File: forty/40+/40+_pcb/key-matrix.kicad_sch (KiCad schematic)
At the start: 48 parts

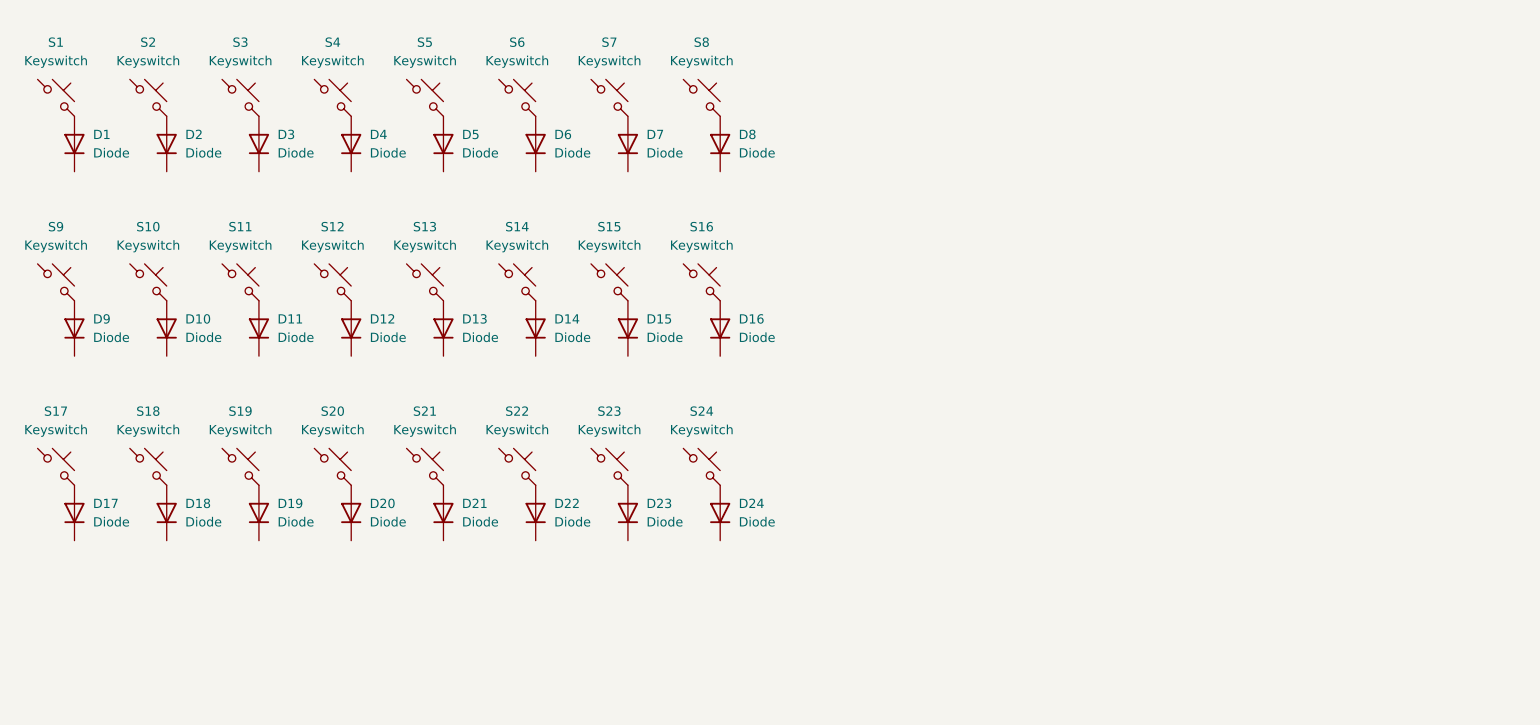
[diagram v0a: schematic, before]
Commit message: macro w/ pcb start
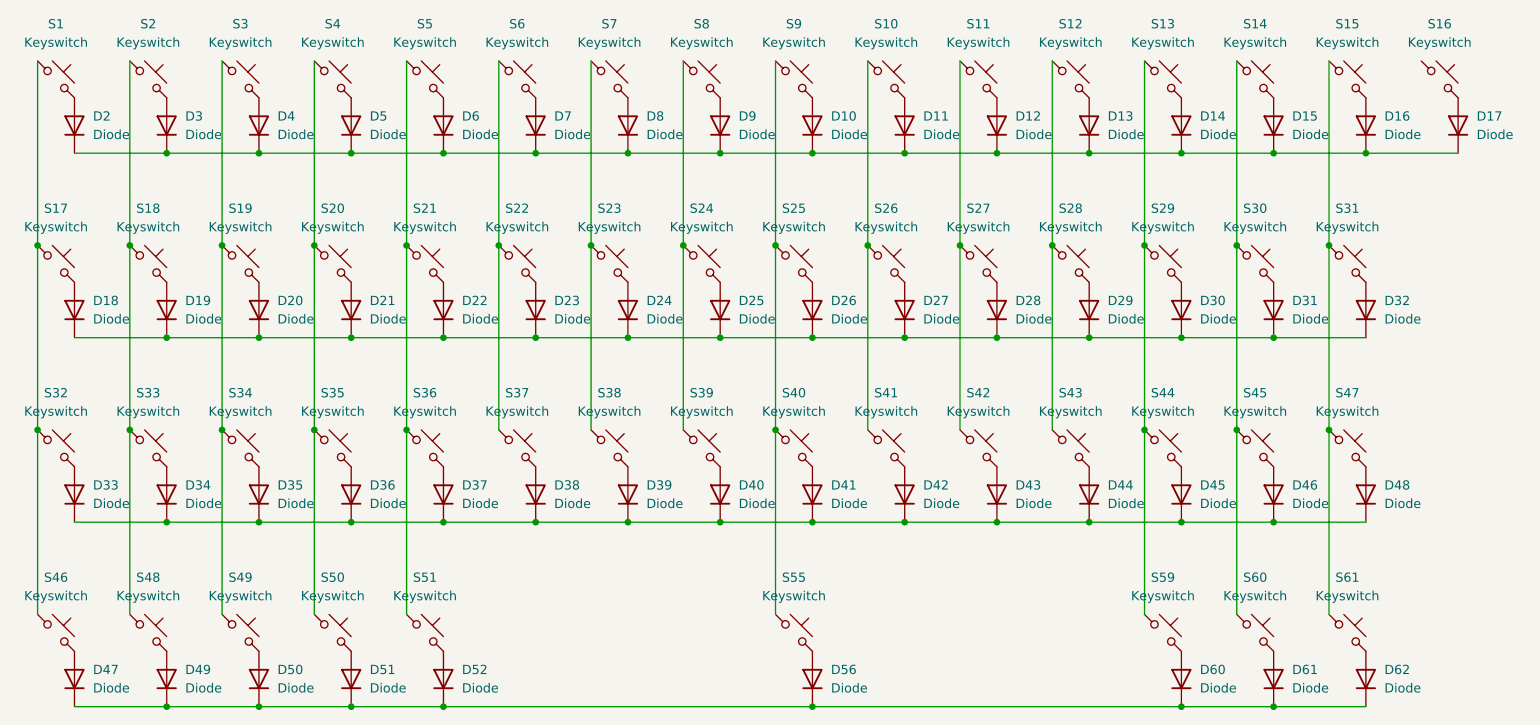
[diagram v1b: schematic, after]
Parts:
- added D26, D27, D28, D29, D30, D31, D32, D33, D34, D35, D36, D37, D38, D39, D40, D41, D42, D43, D44, D45, D46, D47, D48, D49, D50, D51, D52, D56, D60, D61, D62: Diode, symbol ScottoKeebs:Placeholder_Diode
- added S25, S26, S27, S28, S29, S30, S31, S32, S33, S34, S35, S36, S37, S38, S39, S40, S41, S42, S43, S44, S45, S46, S47, S48, S49, S50, S51, S55, S59, S60, S61: Keyswitch, MX_Alps_Hybrid:MX-Alps-Hybrid-1U, symbol ScottoKeebs:Placeholder_Keyswitch
- S1, S10, S11, S12, S13, S14, S15, S16, S17, S18, S19, S2, S20, S21, S22, S23, S24, S3, S4, S5, S6, S7, S8, S9: footprint (none) -> MX_Alps_Hybrid:MX-Alps-Hybrid-1U
- renumbered D9 to D10, D10 to D11, D11 to D12, D12 to D13, D13 to D14, D14 to D15, D15 to D16, D16 to D17, D17 to D18, D18 to D19, D1 to D2, D19 to D20, D20 to D21, D21 to D22, D22 to D23, D23 to D24, D24 to D25, D2 to D3, D3 to D4, D4 to D5, D5 to D6, D6 to D7, D7 to D8, D8 to D9
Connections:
- net at S18.1: now also S2.1, S33.1, S48.1
- net at D5.1 (K): now also D10.1 (K), D11.1 (K), D12.1 (K), D13.1 (K), D14.1 (K), D15.1 (K), D16.1 (K), D17.1 (K), D2.1 (K), D3.1 (K), D4.1 (K), D6.1 (K), D7.1 (K), D8.1 (K), D9.1 (K)
- net at S8.1: now also S24.1, S39.1
- net at S23.1: now also S7.1, S38.1
- net at D18.1 (K): now also D19.1 (K), D20.1 (K), D21.1 (K), D22.1 (K), D23.1 (K), D24.1 (K), D25.1 (K), D26.1 (K), D27.1 (K), D28.1 (K), D29.1 (K), D30.1 (K), D31.1 (K), D32.1 (K)
- net at S15.1: now also S31.1, S47.1, S61.1
- net at S22.1: now also S6.1, S37.1
- net at S14.1: now also S30.1, S45.1, S60.1
- net at S11.1: now also S27.1, S42.1
- net at S10.1: now also S26.1, S41.1
- net at S13.1: now also S29.1, S44.1, S59.1
- net at S1.1: now also S17.1, S32.1, S46.1
- net at S19.1: now also S3.1, S34.1, S49.1
- net at S5.1: now also S21.1, S36.1, S51.1
- net at S9.1: now also S25.1, S40.1, S55.1
- net at S12.1: now also S28.1, S43.1
- net at S20.1: now also S4.1, S35.1, S50.1
- new net: D29.2 (A), S28.2
- new net: D62.2 (A), S61.2
- new net: D45.2 (A), S44.2
- new net: D34.2 (A), S33.2
- new net: D28.2 (A), S27.2
- new net: D33.1 (K), D34.1 (K), D35.1 (K), D36.1 (K), D37.1 (K), D38.1 (K), D39.1 (K), D40.1 (K), D41.1 (K), D42.1 (K), D43.1 (K), D44.1 (K), D45.1 (K), D46.1 (K), D48.1 (K)
- new net: D41.2 (A), S40.2
- new net: D46.2 (A), S45.2
- new net: D30.2 (A), S29.2
- new net: D44.2 (A), S43.2
- new net: D56.2 (A), S55.2
- new net: D43.2 (A), S42.2
- new net: D47.1 (K), D49.1 (K), D50.1 (K), D51.1 (K), D52.1 (K), D56.1 (K), D60.1 (K), D61.1 (K), D62.1 (K)
- new net: D47.2 (A), S46.2
- new net: D37.2 (A), S36.2
- new net: D60.2 (A), S59.2
- new net: D32.2 (A), S31.2
- new net: D35.2 (A), S34.2
- new net: D49.2 (A), S48.2
- new net: D52.2 (A), S51.2
- new net: D31.2 (A), S30.2
- new net: D50.2 (A), S49.2
- new net: D61.2 (A), S60.2
- new net: D36.2 (A), S35.2
- new net: D27.2 (A), S26.2
- new net: D26.2 (A), S25.2
- new net: D33.2 (A), S32.2
- new net: D42.2 (A), S41.2
- new net: D48.2 (A), S47.2
- new net: D38.2 (A), S37.2
- new net: D40.2 (A), S39.2
- new net: D39.2 (A), S38.2
- new net: D51.2 (A), S50.2
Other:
- moved on the sheet: D10, D11, D12, D13, D14, D15, D16, D17, D18, D19, D2, D20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
